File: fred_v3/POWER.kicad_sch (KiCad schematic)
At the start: 4 parts, among them J11 Conn_01x02, U11 AD8001AN, U12 AD8001AN

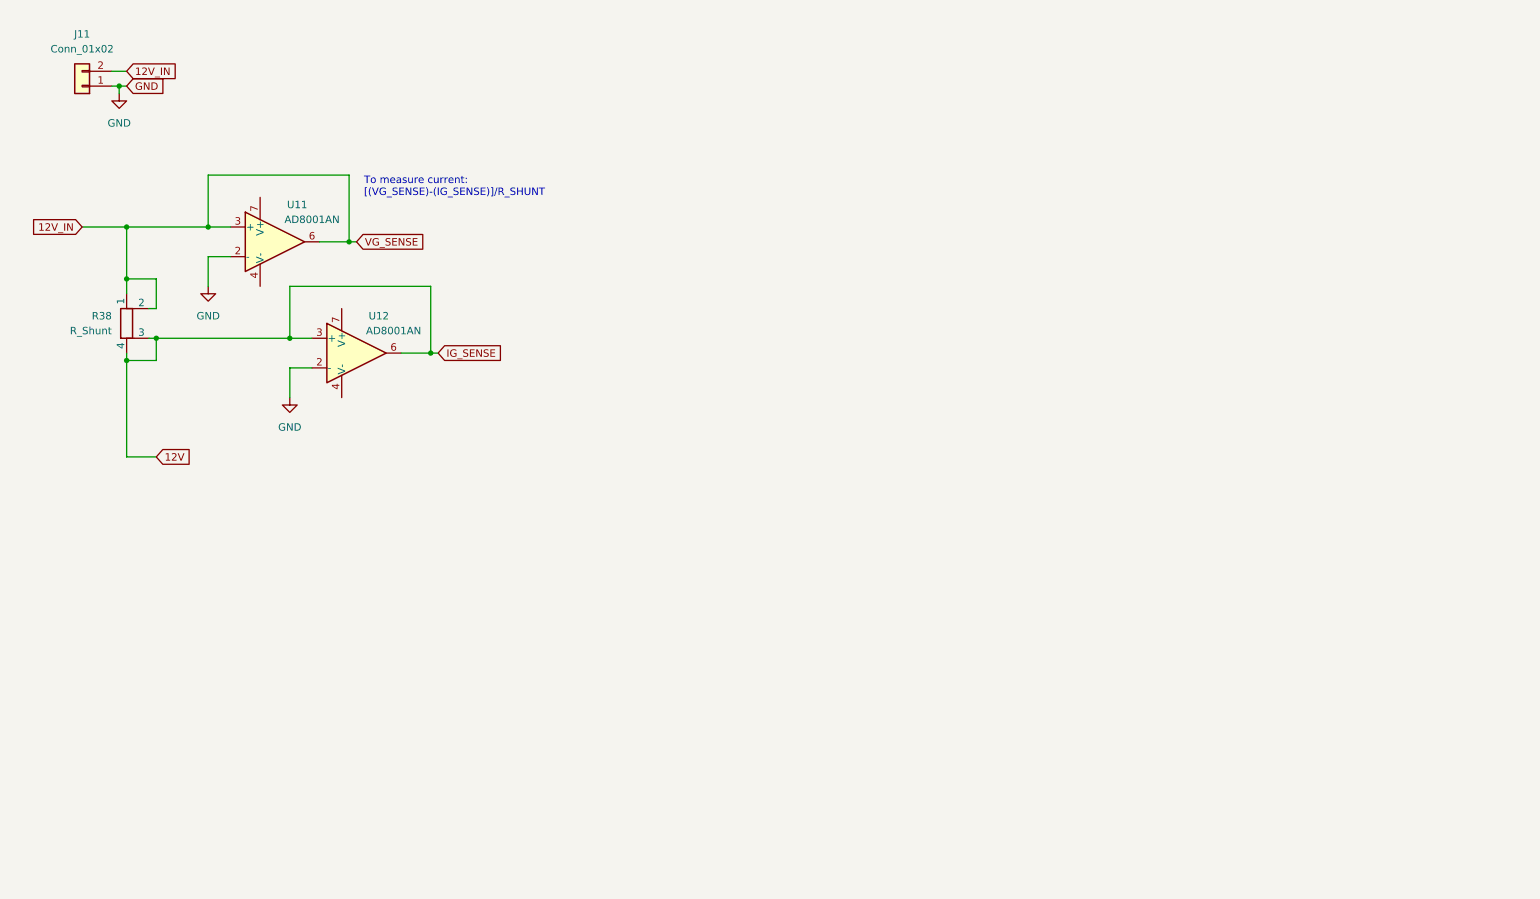
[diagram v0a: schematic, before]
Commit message: Add files via upload
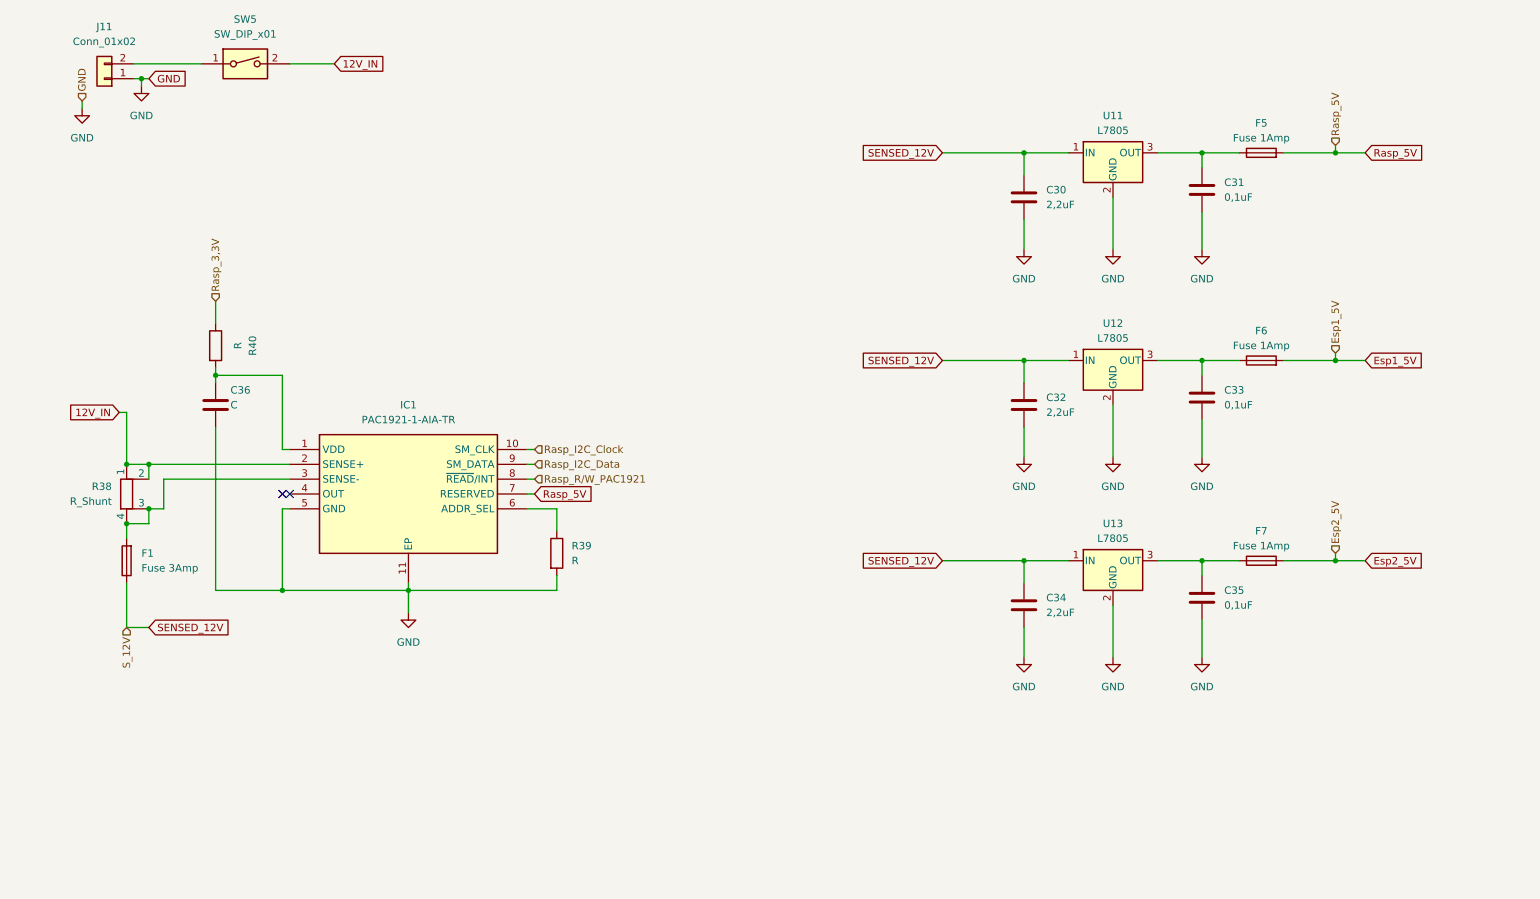
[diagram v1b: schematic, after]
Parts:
- removed U11, U12: AD8001AN, Package_DIP:DIP-8_W7.62mm, symbol Amplifier_Operational:AD8001AN
- added C30, C32, C34: 2,2uF, symbol Device:C
- added C31, C33, C35: 0,1uF, symbol Device:C
- added C36: C, symbol Device:C
- added F1: Fuse 3Amp, symbol Device:Fuse
- added F5, F6, F7: Fuse 1Amp, symbol Device:Fuse
- added IC1: PAC1921-1-AIA-TR, SON50P300X300X90-11N-D, symbol PAC1921:PAC1921-1-AIA-TR
- added R39, R40: R, symbol Device:R
- added SW5: SW_DIP_x01, symbol Switch:SW_DIP_x01
- added U11, U12, U13: L7805, symbol Regulator_Linear:L7805
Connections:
- net 12V_IN: now also IC1.2 (SENSE+), SW5.2; no longer J11.2 (Pin_2)
- net GND: now also C30.2, C31.2, C32.2, C33.2, C34.2, C35.2, C36.2, IC1.11 (EP), IC1.5 (GND), R39.2, U11.2 (GND), U12.2 (GND), U13.2 (GND)
- net 12V: no longer names the net of R38.3, R38.4
- net 12V: now also F1.2, IC1.3 (SENSE-)
- new net: C35.1, F7.1, U13.3 (OUT)
- new net: C31.1, F5.1, U11.3 (OUT)
- new net: C36.1, IC1.1 (VDD), R40.2
- new net: C33.1, F6.1, U12.3 (OUT)
- new net: IC1.6 (ADDR_SEL), R39.1
- new net: J11.2 (Pin_2), SW5.1
- new net Esp1_5V: F6.2
- new net Esp2_5V: F7.2
- new net Rasp_3,3V: R40.1
- new net Rasp_5V: F5.2, IC1.7 (RESERVED)
- new net Rasp_I2C_Clock: IC1.10 (SM_CLK)
- new net Rasp_I2C_Data: IC1.9 (SM_DATA)
- new net Rasp_R/W_PAC1921: IC1.8 (~{READ}/INT)
- new net SENSED_12V: C30.1, C32.1, C34.1, F1.1, U11.1 (IN), U12.1 (IN), U13.1 (IN)
- no-connect marks 0 -> 2
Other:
- note removed: "To measure current: [(VG_SENSE)-(IG_SENSE)]/R_SHUNT"
- moved on the sheet: J11

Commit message: Add files via upload
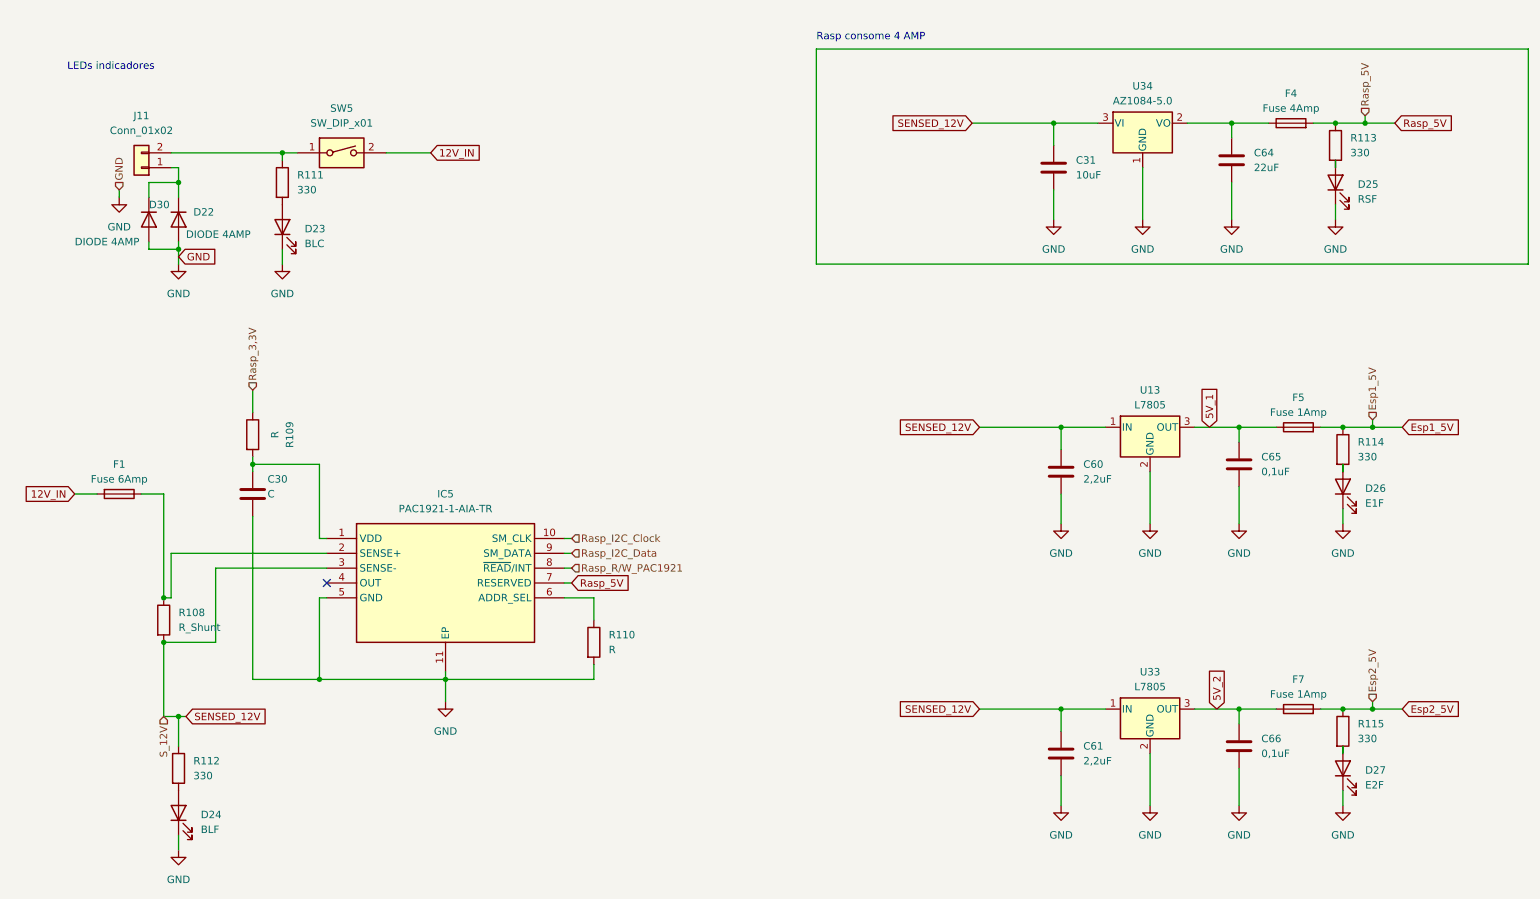
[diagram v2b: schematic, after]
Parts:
- removed C32, C34: 2,2uF, symbol Device:C
- removed C33, C35: 0,1uF, symbol Device:C
- removed C36: C, symbol Device:C
- removed F6: Fuse 1Amp, symbol Device:Fuse
- removed IC1: PAC1921-1-AIA-TR, SON50P300X300X90-11N-D, symbol PAC1921:PAC1921-1-AIA-TR
- removed R38: R_Shunt, symbol Device:R_Shunt
- removed R39, R40: R, symbol Device:R
- removed U11, U12: L7805, symbol Regulator_Linear:L7805
- added C60, C61: 2,2uF, Capacitor_SMD:C_0603_1608Metric_Pad1.08x0.95mm_HandSolder, symbol Device:C
- added C64: 22uF, Capacitor_SMD:C_0603_1608Metric_Pad1.08x0.95mm_HandSolder, symbol Device:C
- added C65, C66: 0,1uF, Capacitor_SMD:C_0603_1608Metric_Pad1.08x0.95mm_HandSolder, symbol Device:C
- added D22, D30: DIODE 4AMP, Diode_THT:D_DO-201AD_P15.24mm_Horizontal, symbol Device:D
- added D23: BLC, LED_SMD:LED_1206_3216Metric_Pad1.42x1.75mm_HandSolder, symbol Device:LED
- added D24: BLF, LED_SMD:LED_1206_3216Metric_Pad1.42x1.75mm_HandSolder, symbol Device:LED
- added D25: RSF, LED_SMD:LED_1206_3216Metric_Pad1.42x1.75mm_HandSolder, symbol Device:LED
- added D26: E1F, LED_SMD:LED_1206_3216Metric_Pad1.42x1.75mm_HandSolder, symbol Device:LED
- added D27: E2F, LED_SMD:LED_1206_3216Metric_Pad1.42x1.75mm_HandSolder, symbol Device:LED
- added F4: Fuse 4Amp, Fuse:Fuseholder_Clip-5x20mm_Littelfuse_111_Inline_P20.00x5.00mm_D1.05mm_Horizontal, symbol Device:Fuse
- added IC5: PAC1921-1-AIA-TR, Package_DFN_QFN:WDFN-10-1EP_3x3mm_P0.5mm_EP1.8x2.5mm, symbol PAC1921:PAC1921-1-AIA-TR
- added R108: R_Shunt, Resistor_SMD:R_0603_1608Metric_Pad0.98x0.95mm_HandSolder, symbol Device:R
- added R109, R110: R, Resistor_SMD:R_0603_1608Metric_Pad0.98x0.95mm_HandSolder, symbol Device:R
- added R111, R112, R113, R114, R115: 330, Resistor_SMD:R_0603_1608Metric_Pad0.98x0.95mm_HandSolder, symbol Device:R
- added U33: L7805, Package_TO_SOT_THT:TO-220-3_Horizontal_TabDown, symbol Regulator_Linear:L7805
- added U34: AZ1084-5.0, Package_TO_SOT_SMD:TO-263-3_TabPin2, symbol Regulator_Linear:AZ1084-5.0
- C30: value 2,2uF -> C; footprint (none) -> Capacitor_SMD:C_0603_1608Metric_Pad1.08x0.95mm_HandSolder
- C31: value 0,1uF -> 10uF; footprint (none) -> Capacitor_SMD:C_0603_1608Metric_Pad1.08x0.95mm_HandSolder
- F1: value Fuse 3Amp -> Fuse 6Amp; footprint (none) -> Fuse:Fuseholder_Clip-5x20mm_Littelfuse_111_Inline_P20.00x5.00mm_D1.05mm_Horizontal
- F5, F7: footprint (none) -> Fuse:Fuseholder_Clip-6.3x32mm_Littelfuse_102_Inline_P34.21x7.62mm_D2.54mm_Horizontal
- J11, SW5: footprint (none) -> Connector_AMASS:AMASS_XT60-M_1x02_P7.20mm_Vertical
- U13: footprint (none) -> Package_TO_SOT_THT:TO-220-3_Horizontal_TabDown
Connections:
- net 12V_IN: now also F1.2
- net Esp1_5V: now also F5.2, R114.1
- net Esp2_5V: now also R115.1
- net GND: now also C60.2, C61.2, C64.2, C65.2, C66.2, D22.2 (A), D23.1 (K), D24.1 (K), D25.1 (K), D26.1 (K), D27.1 (K), D30.2 (A), IC5.11 (EP), IC5.5 (GND), R110.2, U33.2 (GND), U34.1 (GND); no longer J11.1 (Pin_1)
- net Rasp_3,3V: now also R109.1
- net Rasp_5V: now also F4.2, IC5.7 (RESERVED), R113.1; no longer F5.2
- net Rasp_I2C_Clock: now also IC5.10 (SM_CLK)
- net Rasp_I2C_Data: now also IC5.9 (SM_DATA)
- net Rasp_R/W_PAC1921: now also IC5.8 (~{READ}/INT)
- net SENSED_12V: now also C31.1, C60.1, C61.1, IC5.3 (SENSE-), R108.2, R112.1, U33.1 (IN), U34.3 (VI); no longer C30.1, F1.1
- net 5V_1: now reaches U13.3 (OUT)
- net 5V_1: now also F5.1, C65.1; no longer F7.1
- net at J11.2 (Pin_2), SW5.1: now also R111.1
- new net: D27.2 (A), R115.2
- new net: C64.1, F4.1, U34.2 (VO)
- new net: C30.1, IC5.1 (VDD), R109.2
- new net: F1.1, IC5.2 (SENSE+), R108.1
- new net: D26.2 (A), R114.2
- new net: D25.2 (A), R113.2
- new net: IC5.6 (ADDR_SEL), R110.1
- new net: D23.2 (A), R111.2
- new net: D22.1 (K), D30.1 (K), J11.1 (Pin_1)
- new net: D24.2 (A), R112.2
- new net 5V_2: C66.1, F7.1, U33.3 (OUT)
- no-connect marks 2 -> 1
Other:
- note added: "LEDs indicadores"
- note added: "Rasp consome 4 AMP"

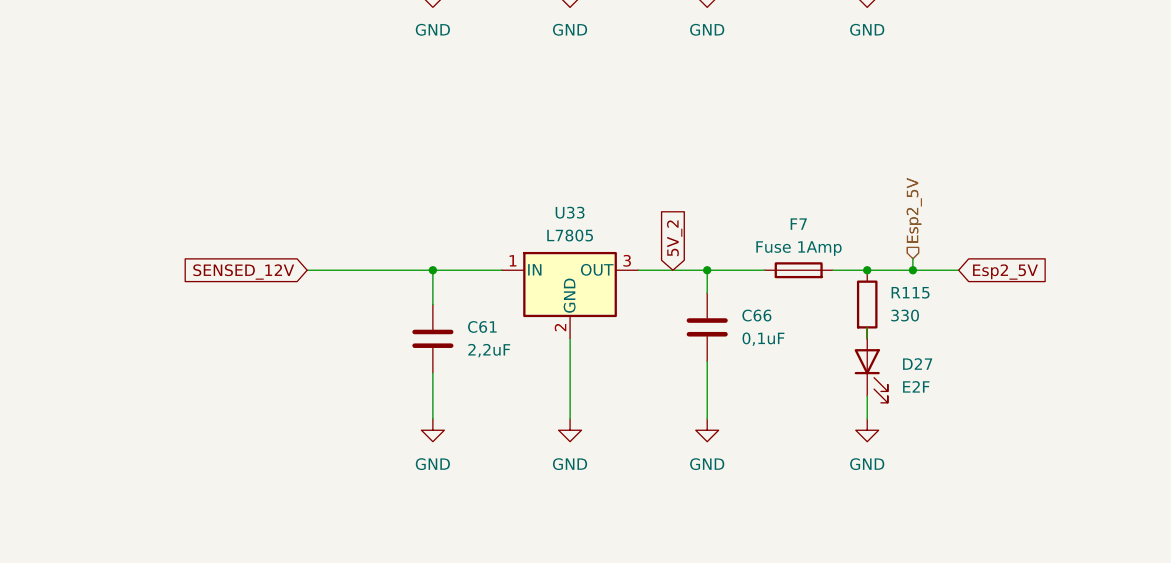
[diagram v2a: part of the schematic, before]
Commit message: Add files via upload
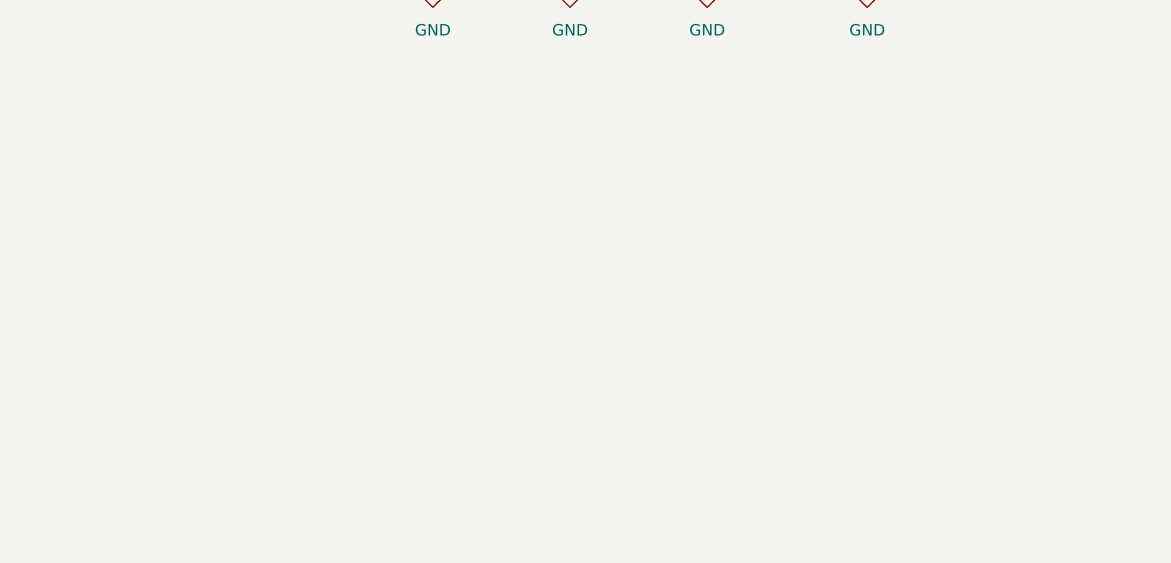
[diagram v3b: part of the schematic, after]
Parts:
- removed C61: 2,2uF, Capacitor_SMD:C_0603_1608Metric_Pad1.08x0.95mm_HandSolder, symbol Device:C
- removed C66: 0,1uF, Capacitor_SMD:C_0603_1608Metric_Pad1.08x0.95mm_HandSolder, symbol Device:C
- removed D27: E2F, LED_SMD:LED_1206_3216Metric_Pad1.42x1.75mm_HandSolder, symbol Device:LED
- removed F7: Fuse 1Amp, Fuse:Fuseholder_Clip-6.3x32mm_Littelfuse_102_Inline_P34.21x7.62mm_D2.54mm_Horizontal, symbol Device:Fuse
- removed R115: 330, Resistor_SMD:R_0603_1608Metric_Pad0.98x0.95mm_HandSolder, symbol Device:R
- removed U33: L7805, Package_TO_SOT_THT:TO-220-3_Horizontal_TabDown, symbol Regulator_Linear:L7805
